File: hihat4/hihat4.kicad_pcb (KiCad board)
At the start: 2 copper layers, 36 parts, among them J1 Input, J2 Input, J3 Output, J4 Power, Q1 BC548, Q2 2N3904, U1 TL074

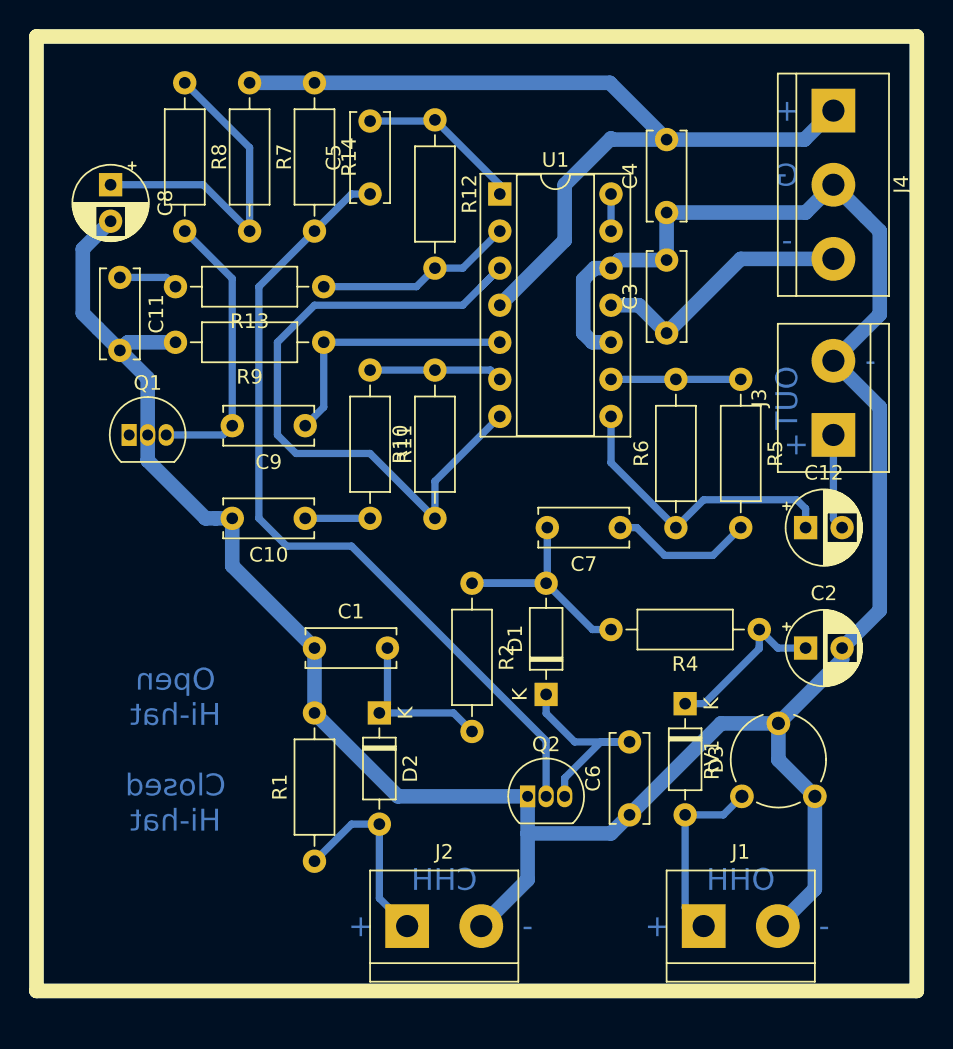
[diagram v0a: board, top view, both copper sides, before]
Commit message: laied out v4
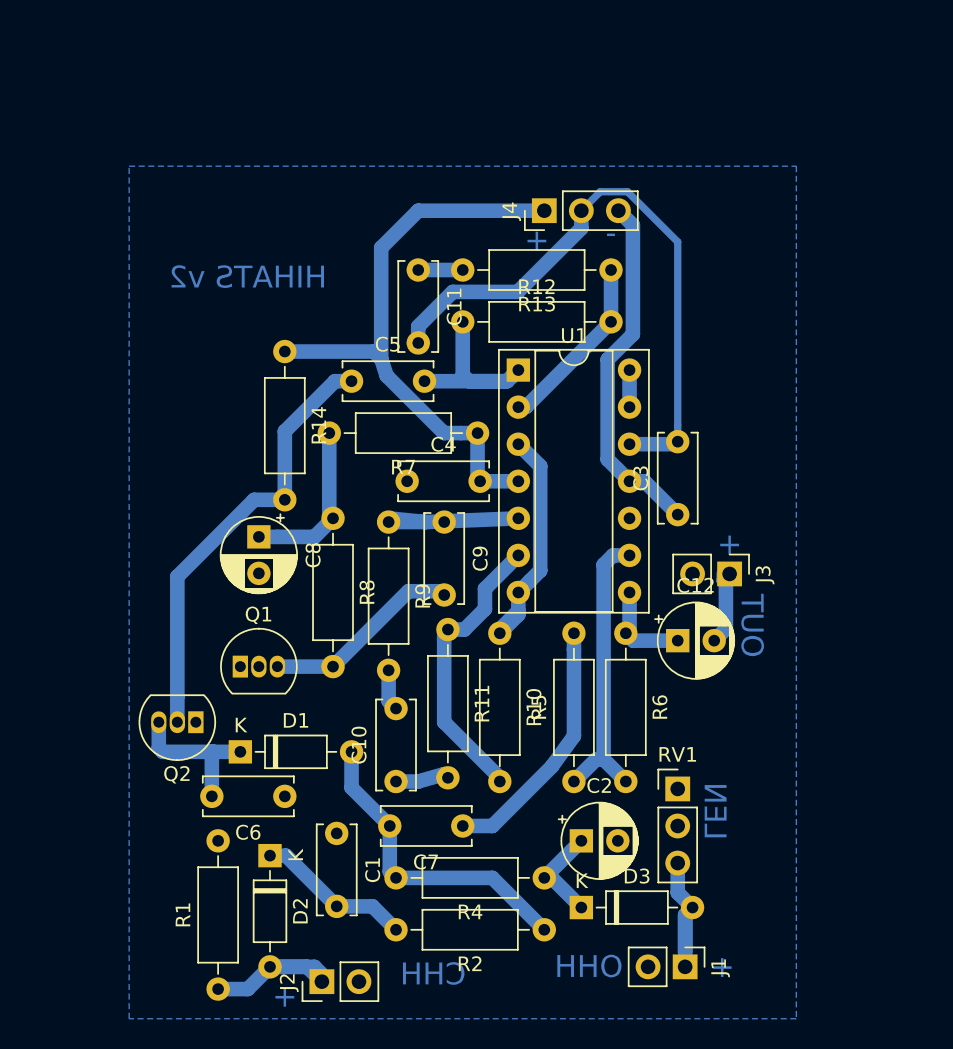
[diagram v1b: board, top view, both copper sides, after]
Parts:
- J1, J2, J3: footprint TerminalBlock:TerminalBlock_bornier-2_P5.08mm -> Connector_PinHeader_2.54mm:PinHeader_1x02_P2.54mm_Vertical
- J4: footprint TerminalBlock:TerminalBlock_bornier-3_P5.08mm -> Connector_PinHeader_2.54mm:PinHeader_1x03_P2.54mm_Vertical
- RV1: footprint Potentiometer_THT:Potentiometer_Piher_PT-6-V_Vertical -> Connector_PinHeader_2.54mm:PinHeader_1x03_P2.54mm_Vertical
- moved R8 31.5 mm to (49.5, 85.1)
- moved R5 29.8 mm to (66.0, 103.1), turned to 90 degrees
- moved R7 28.6 mm to (59.4, 79.2), turned to 180 degrees
- moved C8 26.2 mm to (44.5, 86.4)
- moved C4 25.6 mm to (54.6, 82.5), turned to 0 degrees
- moved R2 24.3 mm to (64.0, 113.3), turned to 180 degrees
- moved C6 23.7 mm to (46.2, 104.1), turned to 180 degrees
- moved Q2 23.3 mm to (40.1, 99.1), turned to 180 degrees
- moved C7 23.1 mm to (58.4, 106.2)
- moved R4 22.5 mm to (64.0, 109.7)
- moved D1 21.3 mm to (43.2, 101.1), turned to 0 degrees
- moved J4 21.0 mm to (64.0, 64.0), turned to 90 degrees
- moved C11 20.5 mm to (55.4, 68.1)
- moved C2 20.3 mm to (66.5, 107.2)
- moved R13 19.7 mm to (68.6, 68.1)
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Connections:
- net +15V renamed +12V
- net -15V renamed -12V
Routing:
- net GND: track 192.3 -> 44.8 mm
- net Net-(R10-Pad1): track 47.5 -> 16.5 mm
- net +12V: track 71.7 -> 41.7 mm
- net Net-(C5-Pad1): track 55.9 -> 30.2 mm
- net Net-(C12-Pad1): track 20.7 -> 6.67 mm
- net Net-(R5-Pad1): track 8.89 -> 20.2 mm
- net Net-(C8-Pad1): track 22.8 -> 11.6 mm
- net Net-(R10-Pad2): track 9.15 -> 19.5 mm
- net Net-(C7-Pad1): track 9.83 -> 17.4 mm
- net Net-(C9-Pad1): track 18.3 -> 11.4 mm
- net -12V: track 18.1 -> 24.5 mm
- net Net-(C9-Pad2): track 19.5 -> 13.6 mm
- net Net-(C2-Pad1): track 11.6 -> 6.97 mm
- net Net-(C6-Pad2): track 14.5 -> 10.9 mm
- net Net-(C5-Pad2): track 11.4 -> 14.3 mm
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- added copper zone on B.Cu, net GND
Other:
- board text added: "HIHATS v2"
- board text added: "LEN"
- board text removed: "G"
- board text removed: "Open Hi-hat Closed Hi-hat"
- board text removed: "POWER"
- board text removed: "Trigger"

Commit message: adjusted output gain 10x, shortened CHH
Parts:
- C1: value 4.7uF -> 100nF
- R1: value 470k -> 100k
- R6: value 1k -> 10k
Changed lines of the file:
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@@
-(kicad_pcb (version 20171130) (host pcbnew "(5.1.5-0)")
+(kicad_pcb (version 20171130) (host pcbnew "(5.0.0)")
   (general
     (thickness 1.6)
@@
   (layers
     (0 F.Cu signal hide)
-    (31 B.Cu signal)
+    (31 B.Cu signal hide)
     (32 B.Adhes user)
     (33 F.Adhes user)
@@
   )
   (setup
-    (last_trace_width 1)
+    (last_trace_width 0.25)
     (user_trace_width 0.5)
     (user_trace_width 1)
@@
     (zone_45_only no)
     (trace_min 0.2)
+    (segment_width 0.2)
+    (edge_width 0.1)
     (via_size 0.8)
     (via_drill 0.4)
@@
     (uvia_min_size 0.2)
     (uvia_min_drill 0.1)
-    (edge_width 0.1)
-    (segment_width 0.2)
     (pcb_text_width 0.3)
     (pcb_text_size 1.5 1.5)
@@
     (pad_to_mask_clearance 0)
     (aux_axis_origin 0 0)
-    (visible_elements FFFFFF7F)
+    (visible_elements 7FFFFFFF)
     (pcbplotparams
       (layerselection 0x010fc_ffffffff)
@@
       (effects (font (size 1 1) (thickness 0.15)))
     )
-    (fp_text value 100k (at 5.08 2.37) (layer F.Fab)
+    (fp_text value 100k (at 10.58 0.872) (layer F.Fab)
       (effects (font (size 1 1) (thickness 0.15)))
     )
@@
       (effects (font (size 1 1) (thickness 0.15)))
     )
-    (fp_text value 100pF (at 2.5 2.5) (layer F.Fab)
+    (fp_text value 100pF (at -2.86 -0.3) (layer F.Fab)
       (effects (font (size 1 1) (thickness 0.15)))
     )
@@
       (effects (font (size 1 1) (thickness 0.15)))
     )
-    (fp_text value 2.2k (at 5.08 2.37) (layer F.Fab)
+    (fp_text value 2.2k (at 0.08 0.822) (layer F.Fab)
       (effects (font (size 1 1) (thickness 0.15)))
     )
@@
       (effects (font (size 1 1) (thickness 0.15)))
     )
-    (fp_text value 100k (at 5.08 2.37 90) (layer F.Fab)
+    (fp_text value 100k (at -0.094 1.09 90) (layer F.Fab)
       (effects (font (size 1 1) (thickness 0.15)))
     )
@@
       (effects (font (size 1 1) (thickness 0.15)))
     )
-    (fp_text value 100k (at 5.08 2.37 90) (layer F.Fab)
+    (fp_text value 100k (at -0.09 1.03 90) (layer F.Fab)
       (effects (font (size 1 1) (thickness 0.15)))
     )
@@
       (effects (font (size 1 1) (thickness 0.15)))
     )
-    (fp_text value 4.7k (at 5.08 2.37) (layer F.Fab)
+    (fp_text value 4.7k (at 0.686 2.248) (layer F.Fab)
       (effects (font (size 1 1) (thickness 0.15)))
     )
@@
       (effects (font (size 1 1) (thickness 0.15)))
     )
-    (fp_text value 1k (at 5.08 2.37 90) (layer F.Fab)
+    (fp_text value 10k (at 6.786 -2.404 90) (layer F.Fab)
       (effects (font (size 1 1) (thickness 0.15)))
     )
@@
       (effects (font (size 1 1) (thickness 0.15)))
     )
-    (fp_text value 1K (at 5.08 2.37 90) (layer F.Fab)
+    (fp_text value 1K (at 2.624 -2.04 90) (layer F.Fab)
       (effects (font (size 1 1) (thickness 0.15)))
     )
@@
       (effects (font (size 1 1) (thickness 0.15)))
     )
-    (fp_text value 470k (at 5.08 2.37 90) (layer F.Fab)
+    (fp_text value 100k (at 5.08 2.37 90) (layer F.Fab)
       (effects (font (size 1 1) (thickness 0.15)))
     )
@@
       (effects (font (size 1 1) (thickness 0.15)))
     )
-    (fp_text value 1N4148 (at 3.81 2.12) (layer F.Fab)
+    (fp_text value 1N4148 (at 5.82 -2.092) (layer F.Fab)
       (effects (font (size 1 1) (thickness 0.15)))
     )
@@
       (effects (font (size 1 1) (thickness 0.15)))
     )
-    (fp_text value 10nF (at 2.5 2.5 90) (layer F.Fab)
+    (fp_text value 10nF (at 3.406 -2.35 90) (layer F.Fab)
       (effects (font (size 1 1) (thickness 0.15)))
     )
@@
       (effects (font (size 1 1) (thickness 0.15)))
     )
-    (fp_text value 470pF (at 2.5 2.5) (layer F.Fab)
+    (fp_text value 470pF (at 2.228 -2.36) (layer F.Fab)
       (effects (font (size 1 1) (thickness 0.15)))
     )
@@
       (effects (font (size 1 1) (thickness 0.15)))
     )
-    (fp_text value 0.47uF (at 2.5 2.5) (layer F.Fab)
+    (fp_text value 0.47uF (at -1.3 -2.192) (layer F.Fab)
       (effects (font (size 1 1) (thickness 0.15)))
     )
@@
       (effects (font (size 1 1) (thickness 0.15)))
     )
-    (fp_text value 4.7uF (at 2.5 2.5 90) (layer F.Fab)
-      (effects (font (size 1 1) (thickness 0.15)))
-    )
+    (fp_text value 100nF (at 2.5 2.5 90) (layer F.Fab)
+      (effects (font (size 1 1) (thickness 0.15)))
+    )
